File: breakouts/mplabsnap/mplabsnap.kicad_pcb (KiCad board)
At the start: 2 copper layers, 26.8 x 35.5 mm, 12 parts, among them J1 USB_A, J2 SNAP, J3 SWD, J4 ISP/UPDI/TPI, J5 UART, J6 Conn_01x04, SW1 5v_3v3_SW, SW2 TPWR, U1 AZ1117CR2-3.3

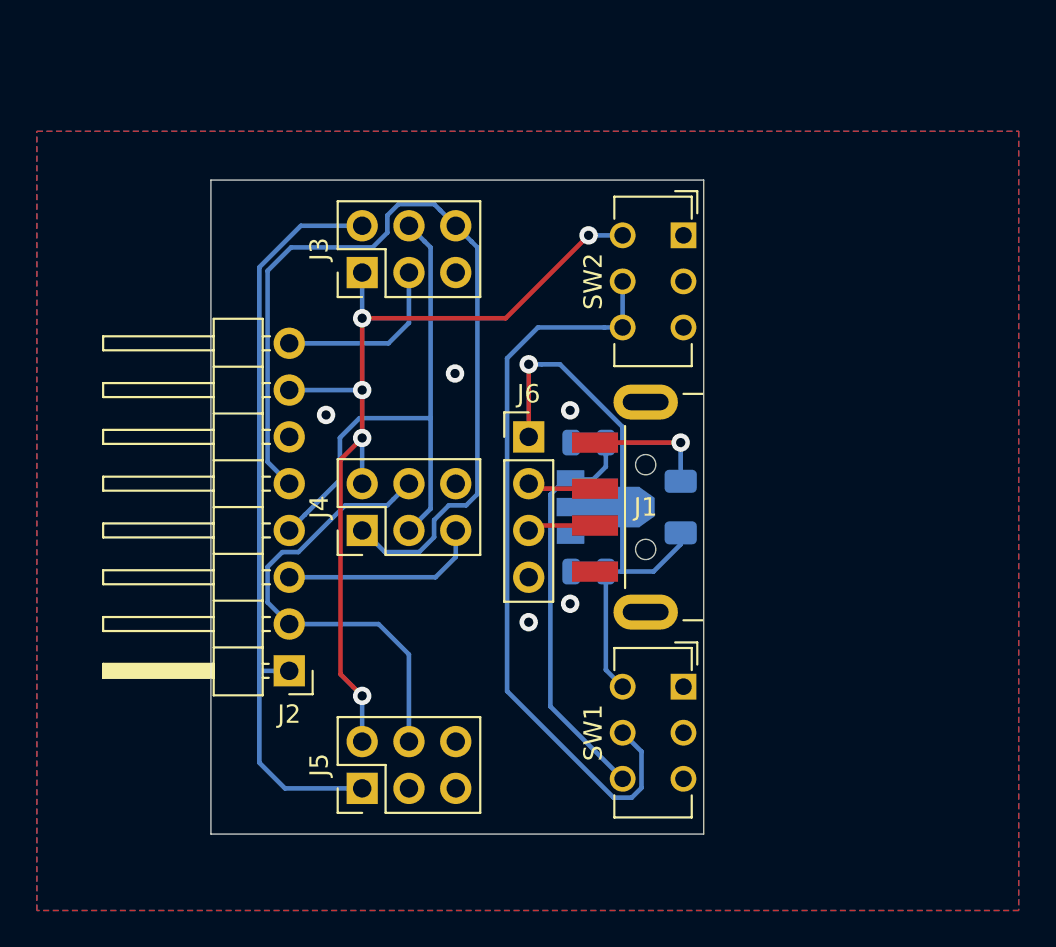
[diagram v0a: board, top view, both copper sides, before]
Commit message: update mplabsnap v2
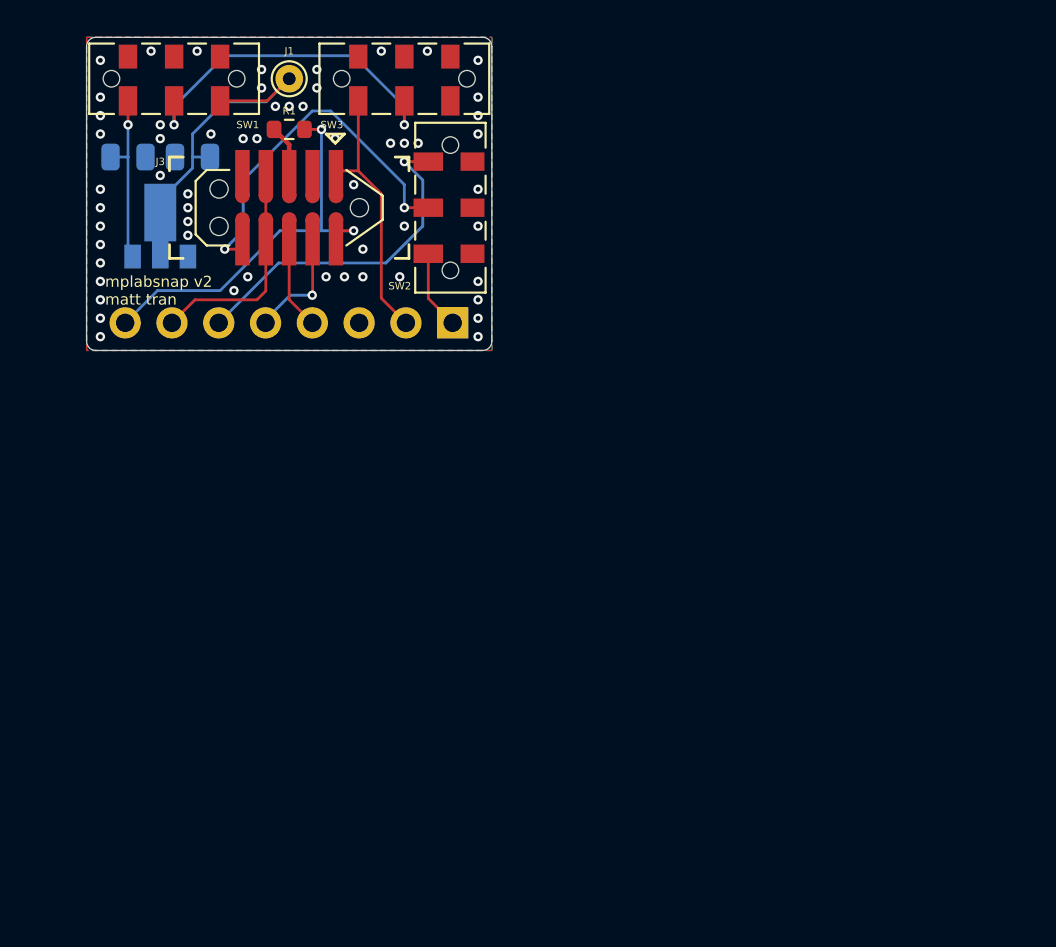
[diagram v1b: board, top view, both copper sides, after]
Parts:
- removed F1: 500mA, Fuse:Fuse_1206_3216Metric
- removed J4: ISP/UPDI/TPI, Connector_PinHeader_2.54mm:PinHeader_2x03_P2.54mm_Vertical
- removed J5: UART, Connector_PinHeader_2.54mm:PinHeader_2x03_P2.54mm_Vertical
- removed J6: Conn_01x04, Connector_PinHeader_2.54mm:PinHeader_1x04_P2.54mm_Vertical
- added R1: 220, Resistor_SMD:R_0603_1608Metric, F.Cu at (150.0, 89.5)
- added SW3: VTG_PWR, extraparts:JS202011JAQN, F.Cu at (156.2, 86.8)
- J1: value USB_A -> 5V; footprint Connector_USB:USB_A_CNCTech_1001-011-01101_Horizontal -> TestPoint:TestPoint_THTPad_D1.5mm_Drill0.7mm
- J2: value SNAP -> snap; footprint Connector_PinHeader_2.54mm:PinHeader_1x08_P2.54mm_Horizontal -> Connector_PinHeader_2.54mm:PinHeader_1x08_P2.54mm_Vertical; moved to B.Cu
- J3: value SWD -> standard; footprint Connector_PinHeader_2.54mm:PinHeader_2x03_P2.54mm_Vertical -> extraparts:TC2050+Header
- SW1: value 5v_3v3_SW -> 5V/3V3; footprint Button_Switch_THT:SW_CuK_JS202011CQN_DPDT_Straight -> extraparts:JS202011JAQN
- SW2: value TPWR -> ~{MCLR}/RST; footprint Button_Switch_THT:SW_CuK_JS202011CQN_DPDT_Straight -> extraparts:JS202011JAQN
- moved SW1 44.0 mm to (143.8, 86.8), turned to 180 degrees
- moved J1 35.1 mm to (150.0, 86.8)
- moved C1 31.1 mm to (144.8, 91.0)
- moved C2 29.4 mm to (141.2, 91.0)
- moved U1 28.2 mm to (143.0, 94.8), turned to 90 degrees
- moved J2 13.4 mm to (158.9, 100.0), turned to 90 degrees
- moved SW2 11.7 mm to (158.8, 93.8), turned to 90 degrees
- moved J3 6.88 mm to (150.0, 93.8), turned to 180 degrees
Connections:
- C2 pad 1: GND -> +3V3
- C2 pad 2: +3V3 -> GND
- J1 pad 1: Net-(F1-Pad2) -> +5V
- J2 pad 1: /SWDIO -> /TVPP
- J2 pad 2: /ISP_MOSI -> VDD
- J2 pad 3: /RESET -> GND
- J2 pad 4: /ISP_SCK -> /PGD
- J2 pad 5: /ISP_MISO -> /PGC
- J2 pad 6: GND -> /TAUX
- J2 pad 7: /VTG -> /TTDI
- J2 pad 8: /MCLR -> /TTMS
- J3 pad 1: /VTG -> VDD
- J3 pad 2: /SWDIO -> /TTMS
- J3 pad 3: /MCLR -> GND
- J3 pad 4: /ISP_SCK -> /PGC
- J3 pad 5: GND -> Net-(J3-Pad5)
- J3 pad 6: /ISP_MISO -> /PGD
- SW1 pad 1: Net-(SW1-Pad1) -> +5V
- SW1 pad 3: Net-(SW1-Pad3) -> +3V3
- SW1 pad 4: +5V -> (no net)
- SW1 pad 5: Net-(SW1-Pad5) -> (no net)
- SW1 pad 6: +3V3 -> (no net)
- SW2 pad 1: Net-(SW2-Pad1) -> /TVPP
- SW2 pad 2: Net-(SW2-Pad2) -> Net-(J3-Pad10)
- SW2 pad 3: Net-(SW2-Pad3) -> /TAUX
- SW2 pad 4: /VTG -> (no net)
- SW2 pad 5: Net-(SW1-Pad5) -> (no net)
- SW2 pad 6: Net-(SW1-Pad5) -> (no net)
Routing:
- net /VTG: track 49.0 -> 0.00 mm, vias 5 -> 0
- net /ISP_MISO: track 48.4 -> 0.00 mm
- net /SWDIO: track 41.2 -> 0.00 mm
- net Net-(SW1-Pad5): track 40.9 -> 0.00 mm
- net /ISP_SCK: track 29.0 -> 0.00 mm
- net /ISP_MOSI: track 25.0 -> 0.00 mm
- net /TTMS: track 0.00 -> 22.5 mm, vias 0 -> 2
- net Net-(J3-Pad10): track 0.00 -> 19.8 mm, vias 0 -> 2
- net Net-(SW1-Pad2): track 0.00 -> 19.4 mm, vias 0 -> 2
- net /TAUX: track 0.00 -> 18.5 mm, vias 0 -> 1
- net +5V: track 34.2 -> 19.3 mm, vias 1 -> 0
- net VDD: track 0.00 -> 14.4 mm
- net +3V3: track 22.0 -> 9.50 mm, vias 0 -> 1
- net /TTDI: track 0.00 -> 12.2 mm
- net /RESET: track 10.9 -> 0.00 mm
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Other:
- board size 26.8 x 35.5 mm -> 22 x 17 mm
- board text added: "5V|3V3"
- board text added: "NC|PWR"
- board text added: "mplabsnap v2 matt tran"
- board text added: "~{RST}|~{MCLR}"
